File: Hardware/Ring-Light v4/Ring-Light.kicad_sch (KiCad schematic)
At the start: 17 parts, among them J1 694106301002, J5 640445-2, Q1 PMOS, U36 TPS62177DQC

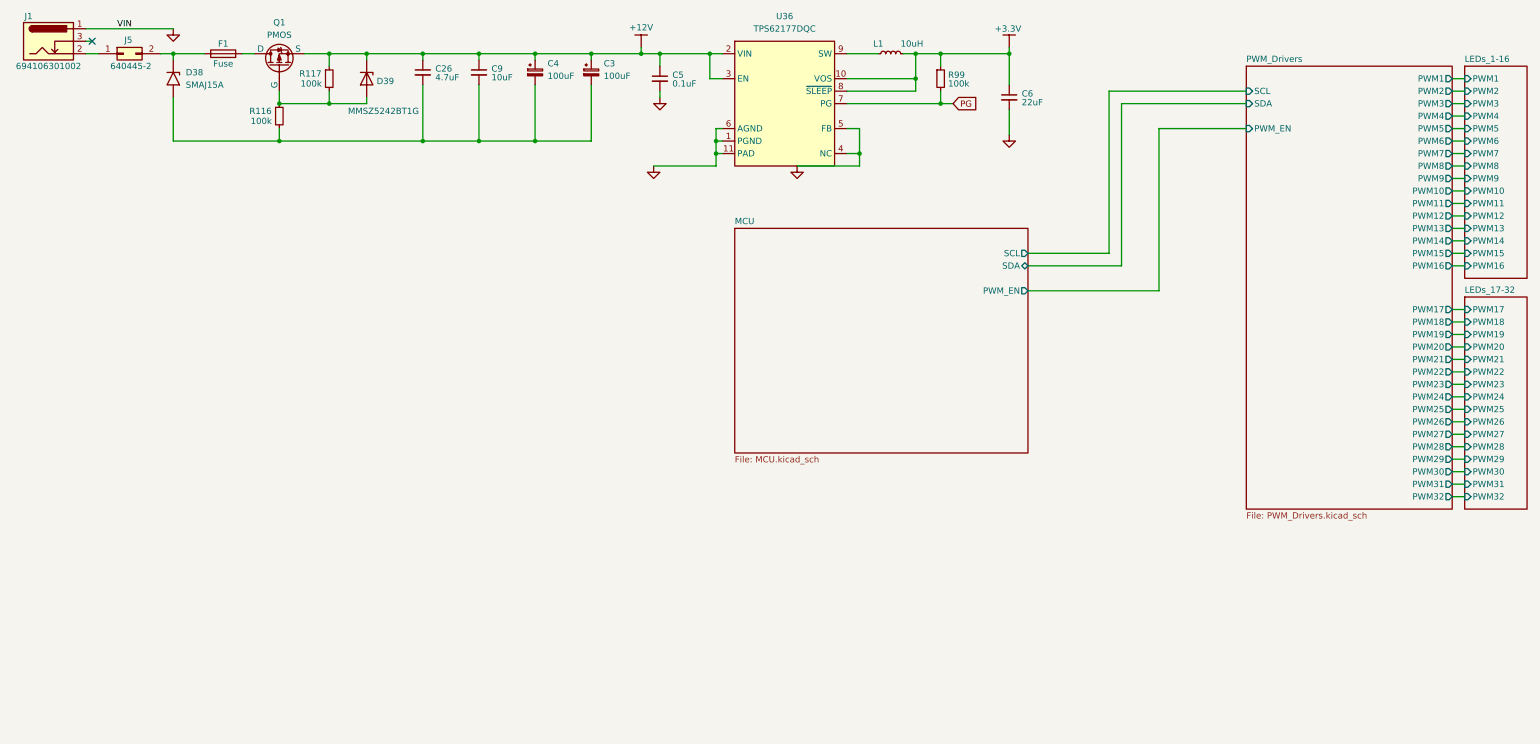
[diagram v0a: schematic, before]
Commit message: m
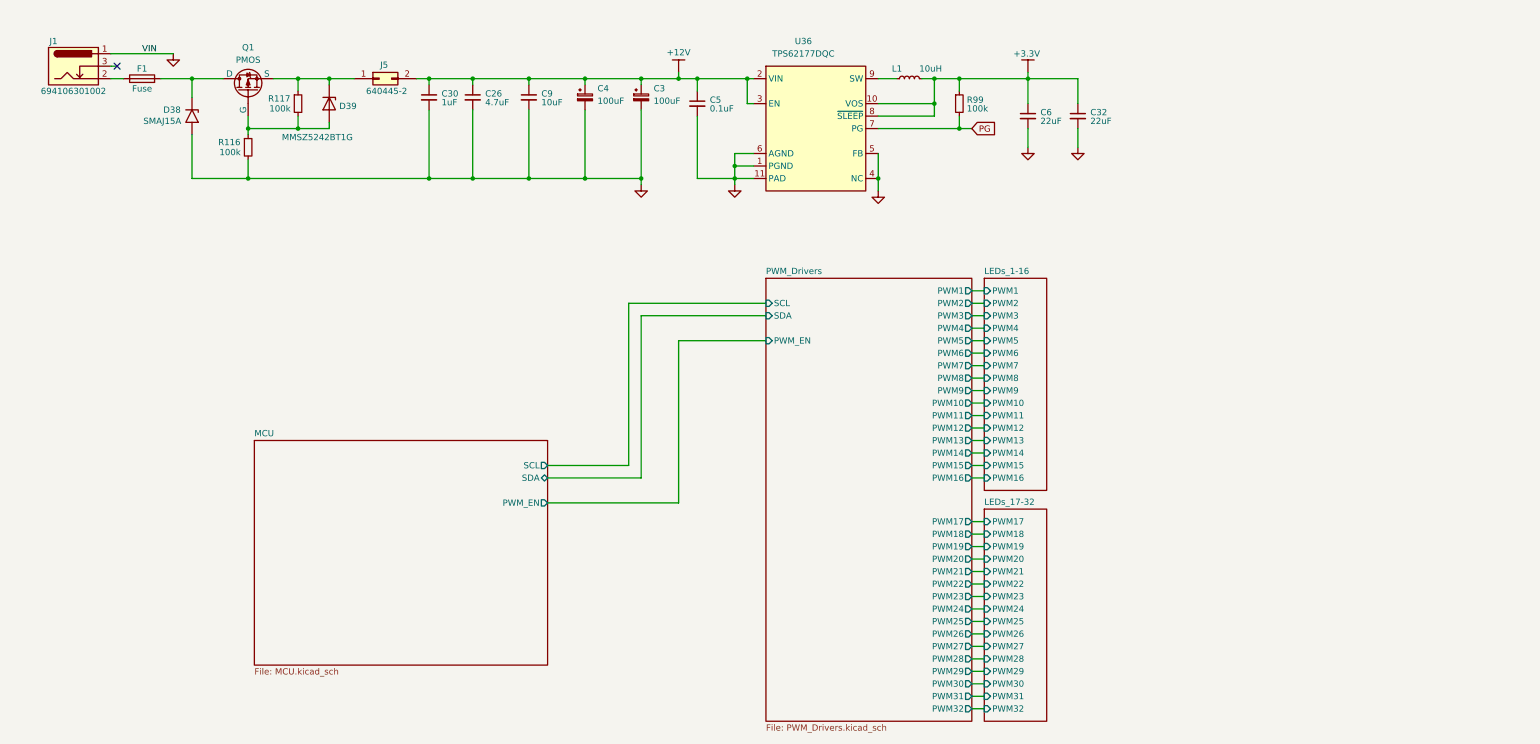
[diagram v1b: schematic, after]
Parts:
- added C30: 1uF, Capacitor_SMD:C_0805_2012Metric, symbol Device:C_Small
- added C32: 22uF, Capacitor_SMD:C_0603_1608Metric, symbol Device:C_Small
- L1: footprint (none) -> Library:WE-LHMI_4020
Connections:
- net +12V: now also J5.2 (Pin_2), C30.1; no longer D39.1 (K), Q1.3 (S), R117.1
- net +3.3V: now also C32.1
- net GND: now also C26.2, C3.2, C4.2, C9.2, D38.2 (A2), R116.2, C30.2, C32.2
- net at J1.2: now also F1.1; no longer J5.1 (Pin_1)
- net at D39.2 (A), R116.1, R117.2: now also Q1.4 (G); no longer Q1.2 (G)
- net at F1.2: now also D38.1 (A1), Q1.5 (D); no longer Q1.1 (D)
- new net: D39.1 (K), J5.1 (Pin_1), Q1.1 (S), Q1.2 (S), Q1.3 (S), R117.1
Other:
- moved on the sheet: C26, C3, C4, C5, C6, C9, D38, D39, F1, J1, J5, L1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
